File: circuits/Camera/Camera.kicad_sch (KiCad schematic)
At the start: 18 parts, among them J2 Conn_01x14_Pin, SW3 SW_SPST, U5 STM32F446RETx, Y1 16MHz

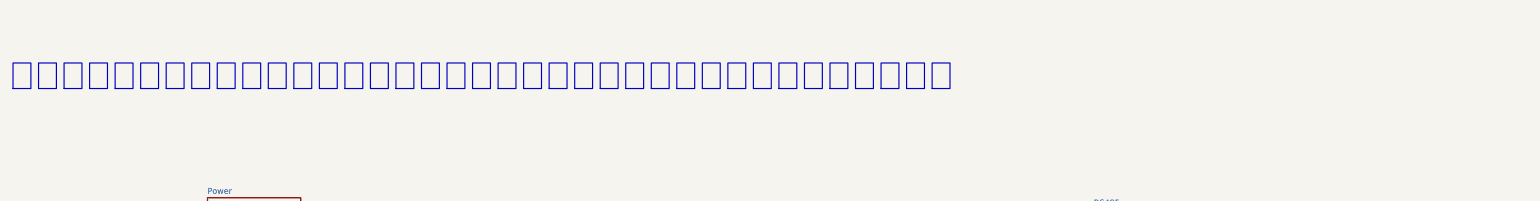
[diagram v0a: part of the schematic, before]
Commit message: 修正
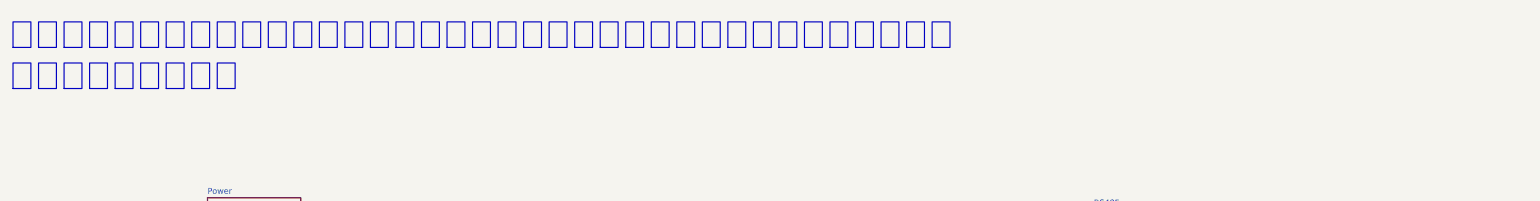
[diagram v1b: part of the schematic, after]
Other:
- note added: "マイコン側のラベルと階層シート側のラベルをそれぞれ対応するように書き換える 電解コンの耐圧注意"
- note removed: "マイコン側のラベルと階層シート側のラベルをそれぞれ対応するように書き換える"
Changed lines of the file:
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@@
     (effects (font (size 1.27 1.27)) (justify left bottom))
   )
-  (text "マイコン側のラベルと階層シート側のラベルをそれぞれ対応するように書き換える" (at 17.78 -5.08 0)
+  (text "マイコン側のラベルと階層シート側のラベルをそれぞれ対応するように書き換える\n電解コンの耐圧注意" (at 17.78 -5.08 0)
     (effects (font (size 5.56 5.56)) (justify left bottom))
   )
